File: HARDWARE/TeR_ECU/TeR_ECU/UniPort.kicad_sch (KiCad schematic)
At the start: 1 part, among them J3 RJ45_Shielded

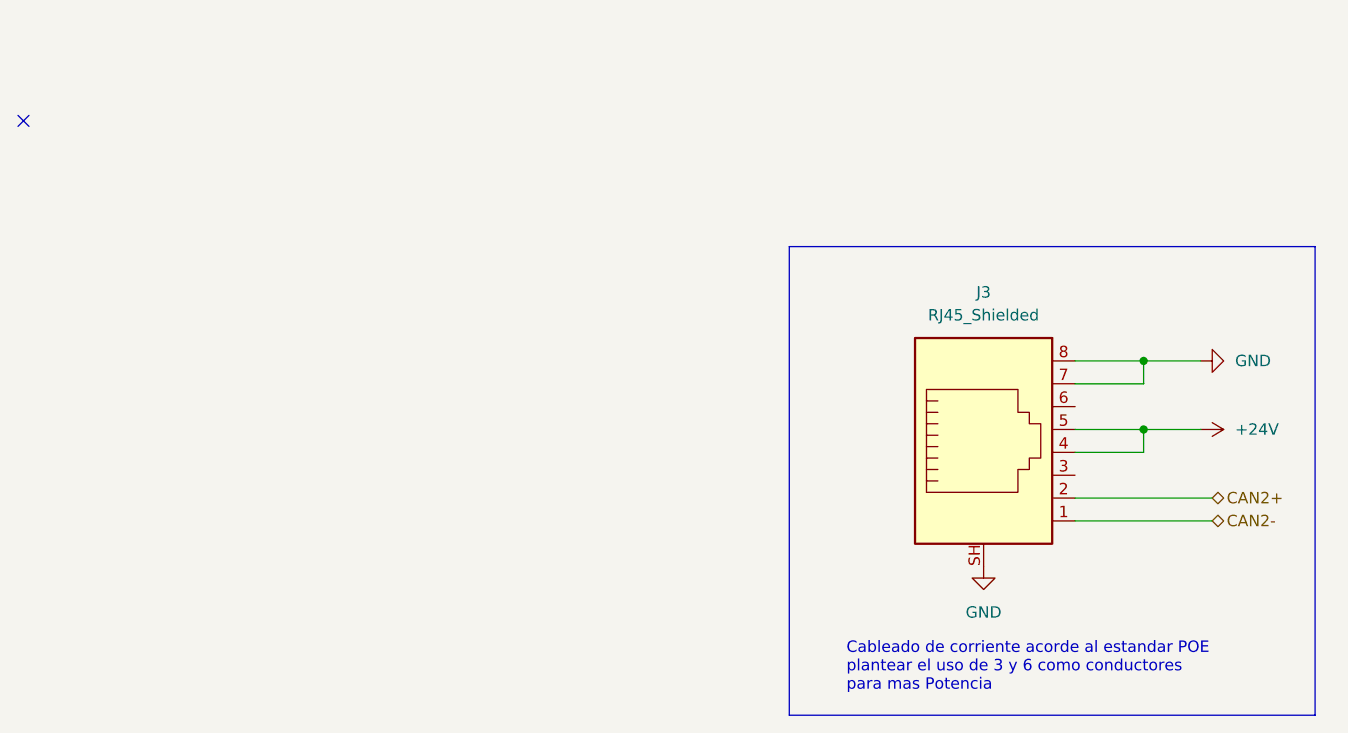
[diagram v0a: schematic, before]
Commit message: Menos el del conector grande, los demas esquematicos acabados
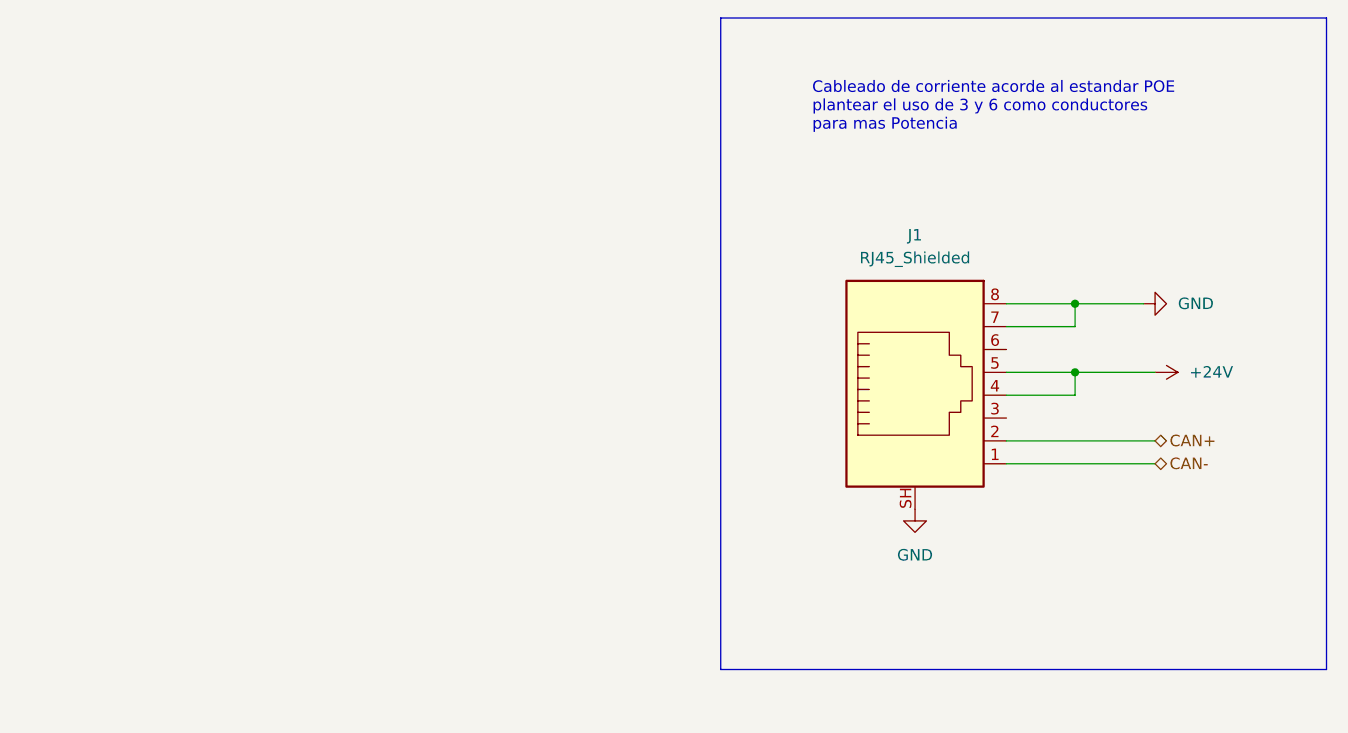
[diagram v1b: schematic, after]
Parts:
- removed J3: RJ45_Shielded, symbol Connector:RJ45_Shielded
- added J1: RJ45_Shielded, symbol Connector:RJ45_Shielded
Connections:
- net +24V: now also J1.4, J1.5
- net GND: now also J1.7, J1.8, J1.SH
- new net CAN+: J1.2
- new net CAN-: J1.1
- no-connect marks 1 -> 0
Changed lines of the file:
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@@
 (kicad_sch (version 20230121) (generator eeschema)
   (paper "A4")
-  (junction (at 152.4 83.82) (diameter 0) (color 0 0 0 0)
+  (junction (at 144.78 85.09) (diameter 0) (color 0 0 0 0)
   )
-  (junction (at 152.4 91.44) (diameter 0) (color 0 0 0 0)
+  (junction (at 144.78 77.47) (diameter 0) (color 0 0 0 0)
   )
-  (no_connect (at 27.94 57.15))
-  (wire (pts (xy 144.78 101.6) (xy 160.02 101.6))
+  (wire (pts (xy 137.16 92.71) (xy 153.67 92.71))
     (stroke (width 0) (type default))
   )
-  (wire (pts (xy 144.78 91.44) (xy 152.4 91.44))
+  (wire (pts (xy 144.78 77.47) (xy 152.4 77.47))
     (stroke (width 0) (type default))
   )
-  (wire (pts (xy 152.4 91.44) (xy 158.75 91.44))
+  (wire (pts (xy 137.16 87.63) (xy 144.78 87.63))
     (stroke (width 0) (type default))
   )
-  (wire (pts (xy 152.4 83.82) (xy 158.75 83.82))
+  (wire (pts (xy 144.78 87.63) (xy 144.78 85.09))
     (stroke (width 0) (type default))
   )
-  (wire (pts (xy 144.78 93.98) (xy 152.4 93.98))
+  (wire (pts (xy 137.16 77.47) (xy 144.78 77.47))
     (stroke (width 0) (type default))
   )
-  (wire (pts (xy 152.4 86.36) (xy 152.4 83.82))
+  (wire (pts (xy 137.16 80.01) (xy 144.78 80.01))
     (stroke (width 0) (type default))
   )
-  (wire (pts (xy 152.4 93.98) (xy 152.4 91.44))
+  (wire (pts (xy 137.16 95.25) (xy 153.67 95.25))
     (stroke (width 0) (type default))
   )
-  (wire (pts (xy 144.78 83.82) (xy 152.4 83.82))
+  (wire (pts (xy 144.78 85.09) (xy 153.67 85.09))
     (stroke (width 0) (type default))
   )
-  (wire (pts (xy 144.78 99.06) (xy 160.02 99.06))
+  (wire (pts (xy 137.16 85.09) (xy 144.78 85.09))
     (stroke (width 0) (type default))
   )
-  (wire (pts (xy 144.78 86.36) (xy 152.4 86.36))
+  (wire (pts (xy 144.78 80.01) (xy 144.78 77.47))
     (stroke (width 0) (type default))
   )
-  (rectangle (start 113.03 71.12) (end 171.45 123.19)
+  (rectangle (start 105.41 45.72) (end 172.72 118.11)
     (stroke (width 0) (type default))
     (fill (type none))
   )
   (text "Cableado de corriente acorde al estandar POE\nplantear el uso de 3 y 6 como conductores\npara mas Potencia\n"
-    (at 119.38 120.65 0)
+    (at 115.57 58.42 0)
     (effects (font (size 1.27 1.27)) (justify left bottom))
   )
-  (hierarchical_label "CAN2+" (shape bidirectional) (at 160.02 99.06 0) (fields_autoplaced)
+  (hierarchical_label "CAN+" (shape bidirectional) (at 153.67 92.71 0) (fields_autoplaced)
     (effects (font (size 1.27 1.27)) (justify left))
   )
-  (hierarchical_label "CAN2-" (shape bidirectional) (at 160.02 101.6 0) (fields_autoplaced)
+  (hierarchical_label "CAN-" (shape bidirectional) (at 153.67 95.25 0) (fields_autoplaced)
     (effects (font (size 1.27 1.27)) (justify left))
   )
-  (symbol (lib_id "power:GND") (at 158.75 83.82 90) (unit 1)
+  (symbol (lib_id "power:+24V") (at 153.67 85.09 270) (unit 1)
     (in_bom yes) (on_board yes) (dnp no) (fields_autoplaced)
-    (property "Reference" "#PWR018" (at 165.1 83.82 0)
+    (property "Reference" "#PWR012" (at 149.86 85.09 0)
       (effects (font (size 1.27 1.27)) hide)
     )
-    (property "Value" "GND" (at 162.56 83.82 90)
-      (effects (font (size 1.27 1.27)) (justify right))
+    (property "Value" "+24V" (at 157.48 85.09 90)
+      (effects (font (size 1.27 1.27)) (justify left))
     )
-    (property "Footprint" "" (at 158.75 83.82 0)
+    (property "Footprint" "" (at 153.67 85.09 0)
       (effects (font (size 1.27 1.27)) hide)
     )
-    (property "Datasheet" "" (at 158.75 83.82 0)
+    (property "Datasheet" "" (at 153.67 85.09 0)
       (effects (font (size 1.27 1.27)) hide)
     )
@@
     (instances
       (project "TeR_ECU"
-        (path "/84413845-c4f3-4743-bcd2-a67649c90902/dd59c3ed-2117-401f-8e0f-5e5867b40ad3"
-          (reference "#PWR018") (unit 1)
+        (path "/84413845-c4f3-4743-bcd2-a67649c90902/c9231e89-0d66-4ea8-9e74-d5a61fdabf8a"
+          (reference "#PWR012") (unit 1)
+        )
+        (path "/84413845-c4f3-4743-bcd2-a67649c90902/89fa6b65-e09d-462b-a9d8-e2037e38fa73"
+          (reference "#PWR039") (unit 1)
+        )
+        (path "/84413845-c4f3-4743-bcd2-a67649c90902/b3d71585-a15b-4975-adfa-12ed469b60dd"
+          (reference "#PWR045") (unit 1)
         )
       )
     )
   )
-  (symbol (lib_id "Connector:RJ45_Shielded") (at 134.62 93.98 0) (unit 1)
+  (symbol (lib_id "power:GND") (at 152.4 77.47 90) (unit 1)
     (in_bom yes) (on_board yes) (dnp no) (fields_autoplaced)
-    (property "Reference" "J3" (at 134.62 76.2 0)
+    (property "Reference" "#PWR011" (at 158.75 77.47 0)
+      (effects (font (size 1.27 1.27)) hide)
+    )
+    (property "Value" "GND" (at 156.21 77.47 90)
+      (effects (font (size 1.27 1.27)) (justify right))
+    )
+    (property "Footprint" "" (at 152.4 77.47 0)
+      (effects (font (size 1.27 1.27)) hide)
+    )
+    (property "Datasheet" "" (at 152.4 77.47 0)
+      (effects (font (size 1.27 1.27)) hide)
+    )
+    (pin "1")
+    (instances
+      (project "TeR_ECU"
+        (path "/84413845-c4f3-4743-bcd2-a67649c90902/c9231e89-0d66-4ea8-9e74-d5a61fdabf8a"
+          (reference "#PWR011") (unit 1)
+        )
+        (path "/84413845-c4f3-4743-bcd2-a67649c90902/89fa6b65-e09d-462b-a9d8-e2037e38fa73"
+          (reference "#PWR019") (unit 1)
+        )
+        (path "/84413845-c4f3-4743-bcd2-a67649c90902/b3d71585-a15b-4975-adfa-12ed469b60dd"
+          (reference "#PWR043") (unit 1)
+        )
+      )
+    )
+  )
+  (symbol (lib_id "power:GND") (at 127 100.33 0) (unit 1)
+    (in_bom yes) (on_board yes) (dnp no) (fields_autoplaced)
+    (property "Reference" "#PWR013" (at 127 106.68 0)
+      (effects (font (size 1.27 1.27)) hide)
+    )
+    (property "Value" "GND" (at 127 105.41 0)
       (effects (font (size 1.27 1.27)))
     )
-    (property "Value" "RJ45_Shielded" (at 134.62 78.74 0)
+    (property "Footprint" "" (at 127 100.33 0)
+      (effects (font (size 1.27 1.27)) hide)
+    )
+    (property "Datasheet" "" (at 127 100.33 0)
+      (effects (font (size 1.27 1.27)) hide)
+    )
+    (pin "1")
+    (instances
+      (project "TeR_ECU"
+        (path "/84413845-c4f3-4743-bcd2-a67649c90902/c9231e89-0d66-4ea8-9e74-d5a61fdabf8a"
+          (reference "#PWR013") (unit 1)
+        )
+        (path "/84413845-c4f3-4743-bcd2-a67649c90902/89fa6b65-e09d-462b-a9d8-e2037e38fa73"
+          (reference "#PWR017") (unit 1)
+        )
+        (path "/84413845-c4f3-4743-bcd2-a67649c90902/b3d71585-a15b-4975-adfa-12ed469b60dd"
+          (reference "#PWR041") (unit 1)
+        )
+      )
+    )
+  )
+  (symbol (lib_id "Connector:RJ45_Shielded") (at 127 87.63 0) (unit 1)
+    (in_bom yes) (on_board yes) (dnp no) (fields_autoplaced)
+    (property "Reference" "J1" (at 127 69.85 0)
       (effects (font (size 1.27 1.27)))
     )
-    (property "Footprint" "" (at 134.62 93.345 90)
+    (property "Value" "RJ45_Shielded" (at 127 72.39 0)
+      (effects (font (size 1.27 1.27)))
+    )
+    (property "Footprint" "" (at 127 86.995 90)
       (effects (font (size 1.27 1.27)) hide)
     )
-    (property "Datasheet" "~" (at 134.62 93.345 90)
+    (property "Datasheet" "~" (at 127 86.995 90)
       (effects (font (size 1.27 1.27)) hide)
     )
@@
     (instances
       (project "TeR_ECU"
-        (path "/84413845-c4f3-4743-bcd2-a67649c90902/dd59c3ed-2117-401f-8e0f-5e5867b40ad3"
+        (path "/84413845-c4f3-4743-bcd2-a67649c90902/c9231e89-0d66-4ea8-9e74-d5a61fdabf8a"
+          (reference "J1") (unit 1)
+        )
+        (path "/84413845-c4f3-4743-bcd2-a67649c90902/89fa6b65-e09d-462b-a9d8-e2037e38fa73"
+          (reference "J2") (unit 1)
+        )
+        (path "/84413845-c4f3-4743-bcd2-a67649c90902/b3d71585-a15b-4975-adfa-12ed469b60dd"
           (reference "J3") (unit 1)
         )
       )
-    )
-  )
-  (symbol (lib_id "power:+24V") (at 158.75 91.44 270) (unit 1)
-    (in_bom yes) (on_board yes) (dnp no) (fields_autoplaced)
-    (property "Reference" "#PWR017" (at 154.94 91.44 0)
-      (effects (font (size 1.27 1.27)) hide)
-    )
-    (property "Value" "+24V" (at 162.56 91.44 90)
-      (effects (font (size 1.27 1.27)) (justify left))
-    )
-    (property "Footprint" "" (at 158.75 91.44 0)
-      (effects (font (size 1.27 1.27)) hide)
-    )
-    (property "Datasheet" "" (at 158.75 91.44 0)
-      (effects (font (size 1.27 1.27)) hide)
-    )
-    (pin "1")
-    (instances
-      (project "TeR_ECU"
-        (path "/84413845-c4f3-4743-bcd2-a67649c90902/dd59c3ed-2117-401f-8e0f-5e5867b40ad3"
-          (reference "#PWR017") (unit 1)
-        )
-      )
-    )
-  )
-  (symbol (lib_id "power:GND") (at 134.62 106.68 0) (unit 1)
-    (in_bom yes) (on_board yes) (dnp no) (fields_autoplaced)
-    (property "Reference" "#PWR019" (at 134.62 113.03 0)
-      (effects (font (size 1.27 1.27)) hide)
-    )
-    (property "Value" "GND" (at 134.62 111.76 0)
-      (effects (font (size 1.27 1.27)))
-    )
-    (property "Footprint" "" (at 134.62 106.68 0)
-      (effects (font (size 1.27 1.27)) hide)
-    )
-    (property "Datasheet" "" (at 134.62 106.68 0)
-      (effects (font (size 1.27 1.27)) hide)
-    )
-    (pin "1")
-    (instances
-      (project "TeR_ECU"
-        (path "/84413845-c4f3-4743-bcd2-a67649c90902/dd59c3ed-2117-401f-8e0f-5e5867b40ad3"
-          (reference "#PWR019") (unit 1)
-        )
-      )
